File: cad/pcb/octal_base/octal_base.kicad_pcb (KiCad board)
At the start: 2 copper layers, 23.6 x 23.6 mm, 13 parts, among them J1 Octal Base, J2 Pin Socket

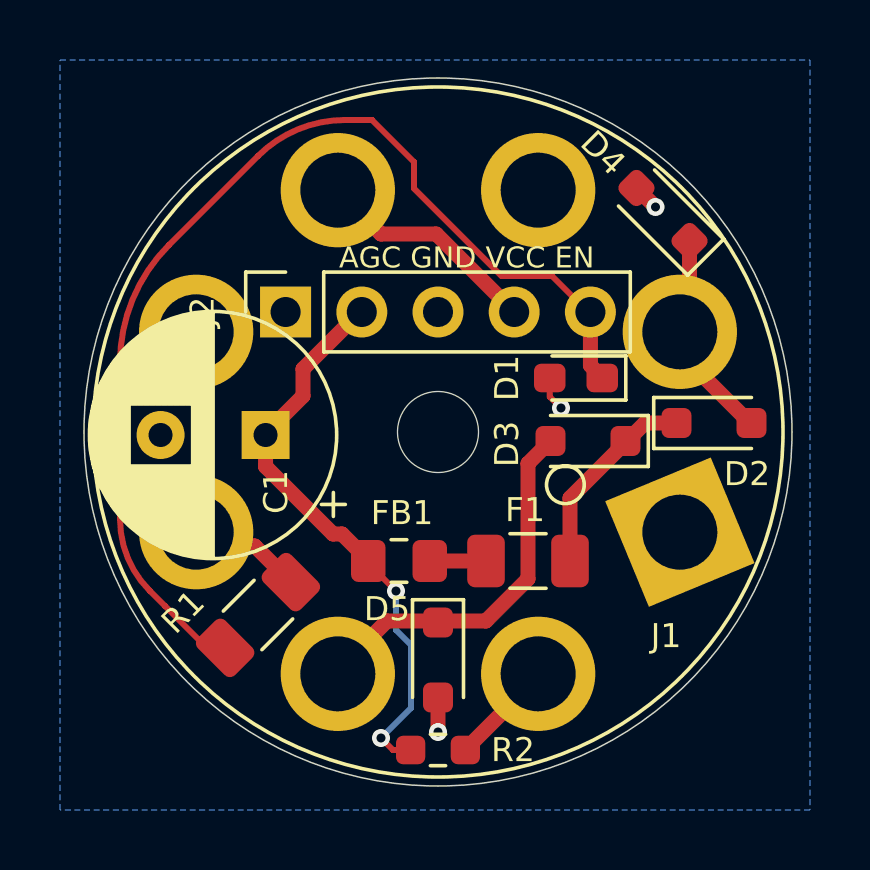
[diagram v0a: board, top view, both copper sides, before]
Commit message: Add: Base Cleanup
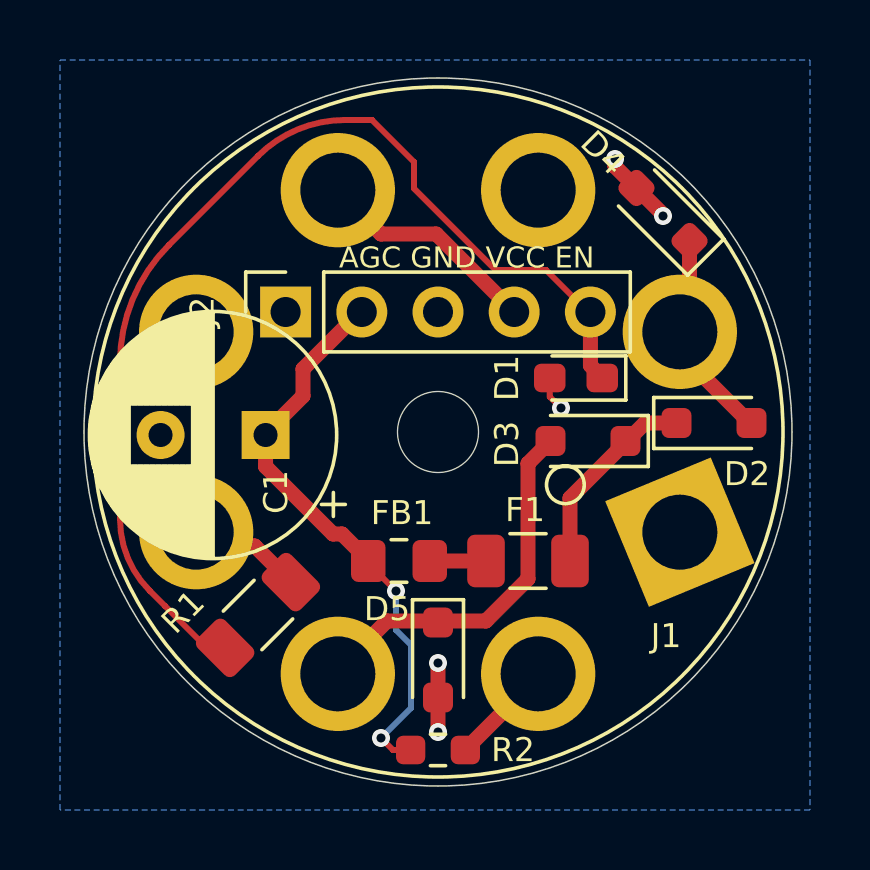
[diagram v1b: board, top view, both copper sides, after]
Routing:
- net GND: track 3.20 -> 6.02 mm, vias 3 -> 5
